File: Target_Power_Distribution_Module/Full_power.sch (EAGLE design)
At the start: 28 parts, among them IC1 MCP1702, Q1 NFET, Q2 PFET, Q3 NFET, Q4 PFET

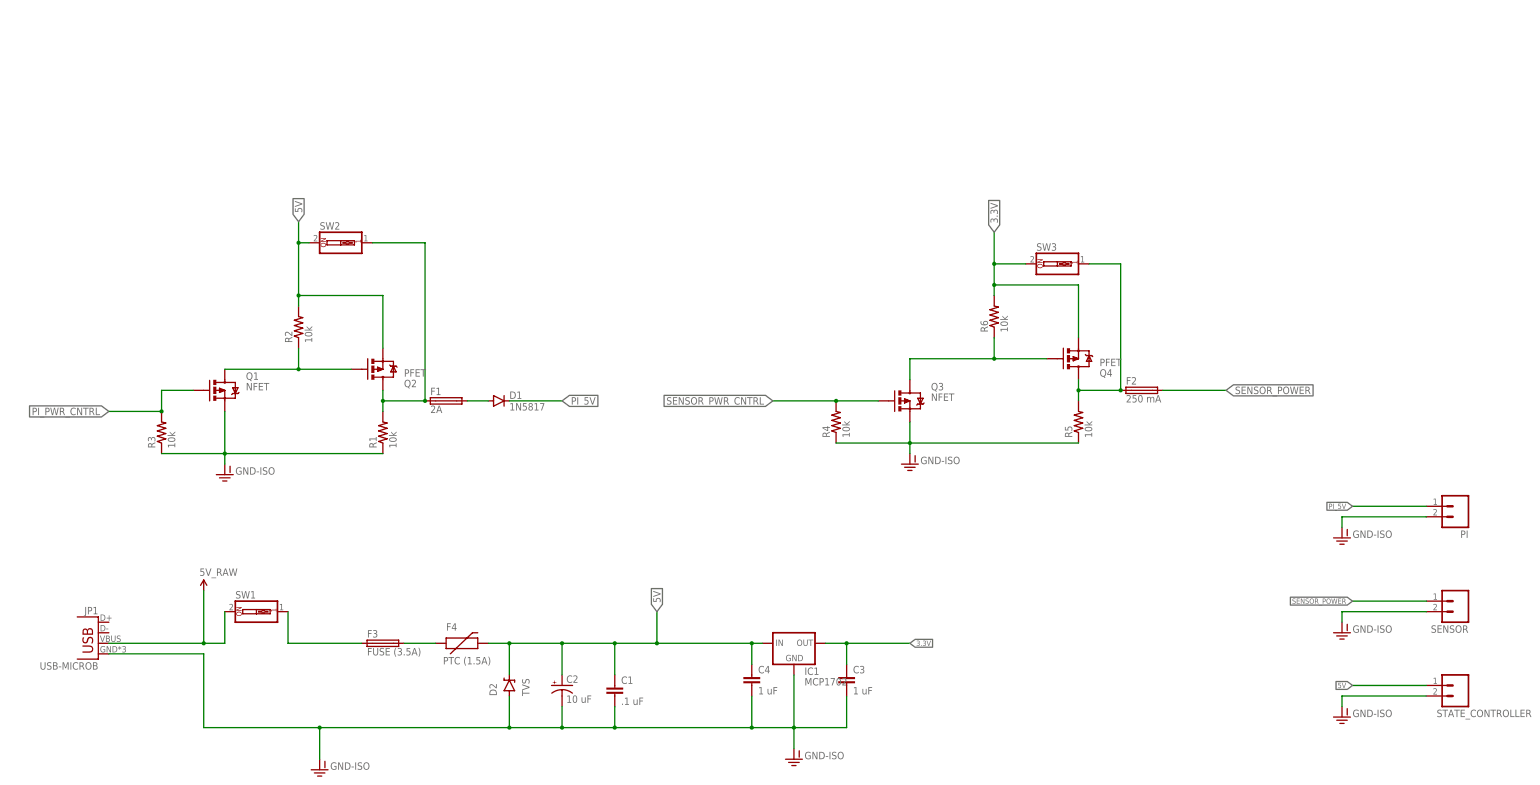
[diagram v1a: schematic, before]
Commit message: Some schematic updates
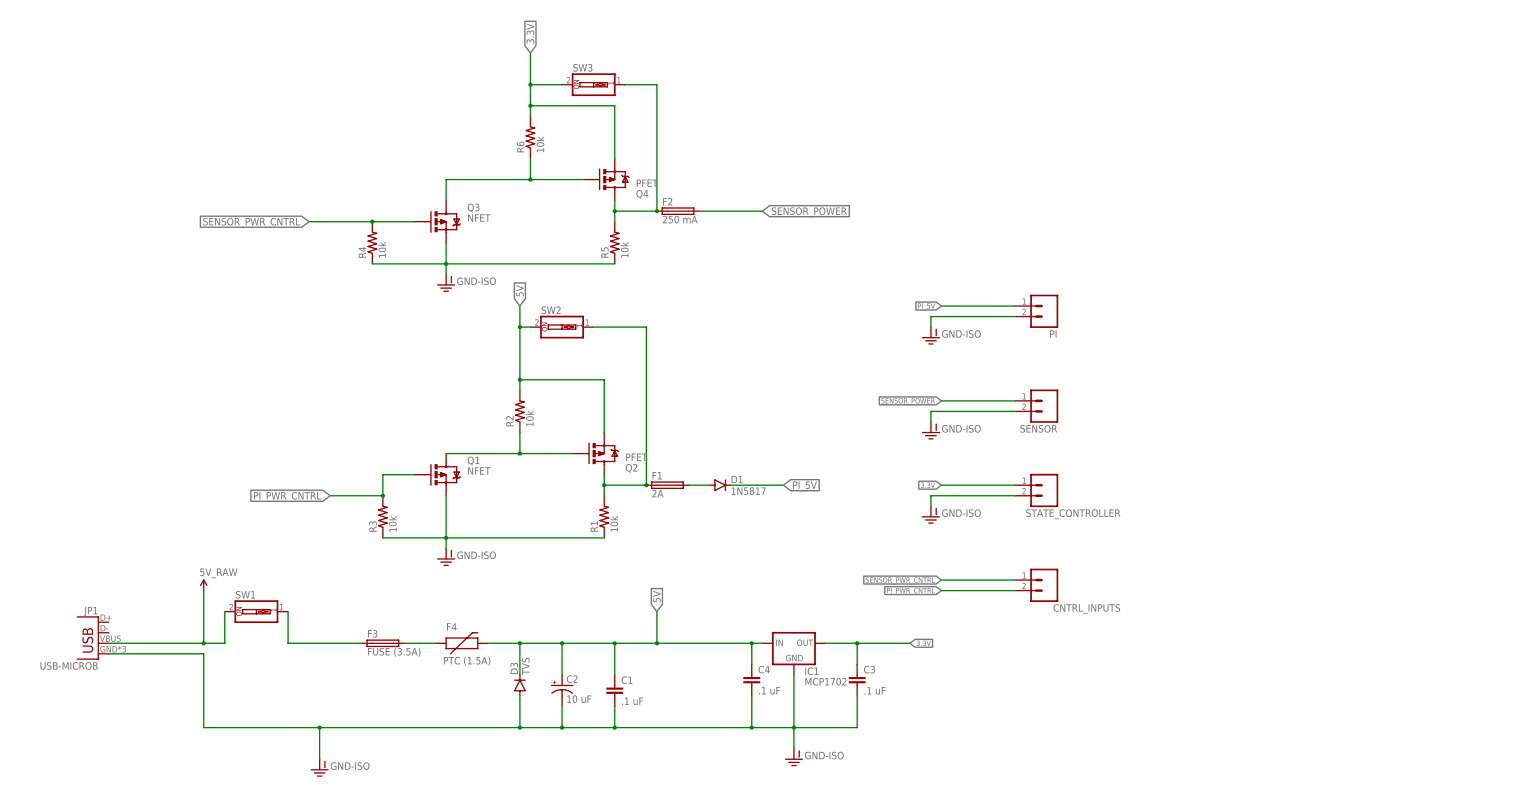
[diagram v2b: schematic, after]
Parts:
- removed D2: TVS, SparkFun-DiscreteSemi:DIODE-ZENERPTH
- added CNTRL_INPUTS: (no value), SparkFun-Connectors:M02PTH
- added D3: TVS, SparkFun-DiscreteSemi:DIODEPTH
- C3, C4: value 1 uF -> .1 uF
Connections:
- net 3.3V: now also STATE_CONTROLLER.1
- net 5V: now also D3.C; no longer D2.C, STATE_CONTROLLER.1
- net GND-ISO: now also D3.A; no longer D2.A
- net PI_PWR_CNTRL: now also CNTRL_INPUTS.2
- net SENSOR_PWR_CNTRL: now also CNTRL_INPUTS.1
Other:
- moved on the sheet: C3, D1, F1, F2, PI, Q1, Q2, Q3, Q4, R1, R2, R3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
